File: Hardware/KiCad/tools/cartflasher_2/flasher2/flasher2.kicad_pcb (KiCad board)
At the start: 4 copper layers, 89 x 93 mm, 32 parts, among them J1 USB_C_Receptacle_USB2.0, J2 ICSP, J3 ICSP, SW1 SW_Push, U2 AVR64DA64-I/PT, U3 FT232RL

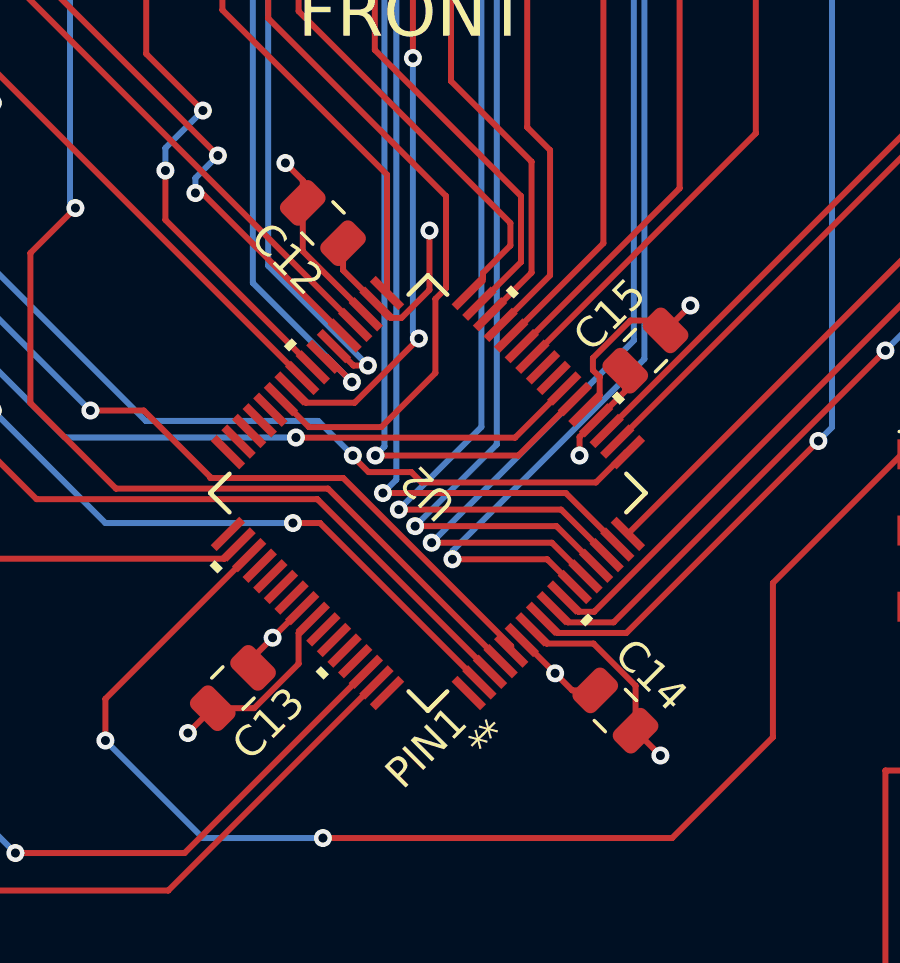
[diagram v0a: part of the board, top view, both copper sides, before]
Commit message: collect production documents for quoting
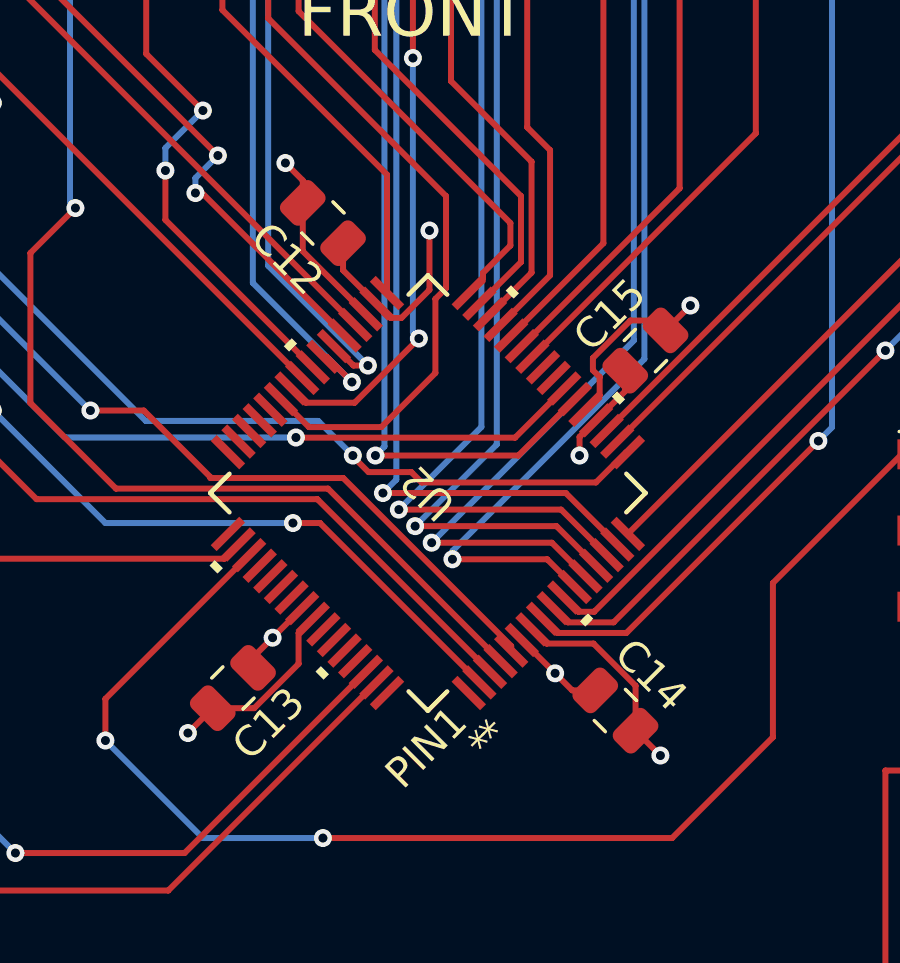
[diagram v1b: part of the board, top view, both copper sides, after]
